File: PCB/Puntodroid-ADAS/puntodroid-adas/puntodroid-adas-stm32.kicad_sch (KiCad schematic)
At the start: 23 parts, among them J1 USB_B, J2 BOOTLOADER, J3 SWD PROGRAMMER, U1 STM32F446VETx, U2 CM1293A, Y1 16MHz

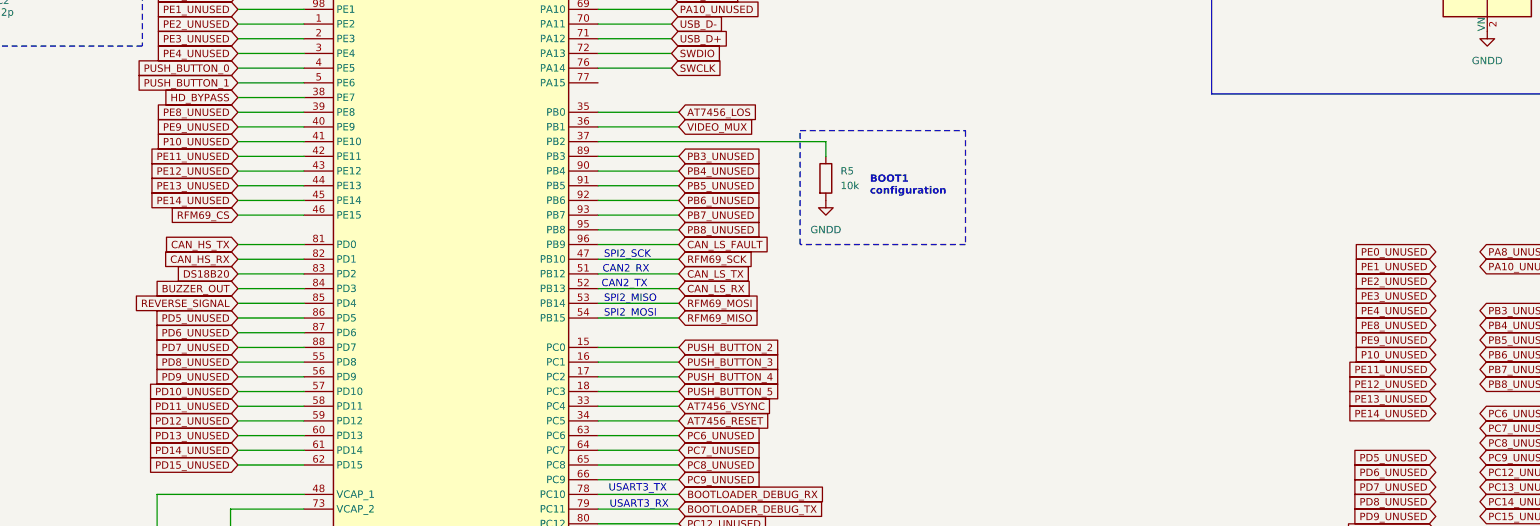
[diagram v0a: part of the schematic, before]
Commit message: update puntodroid schematic
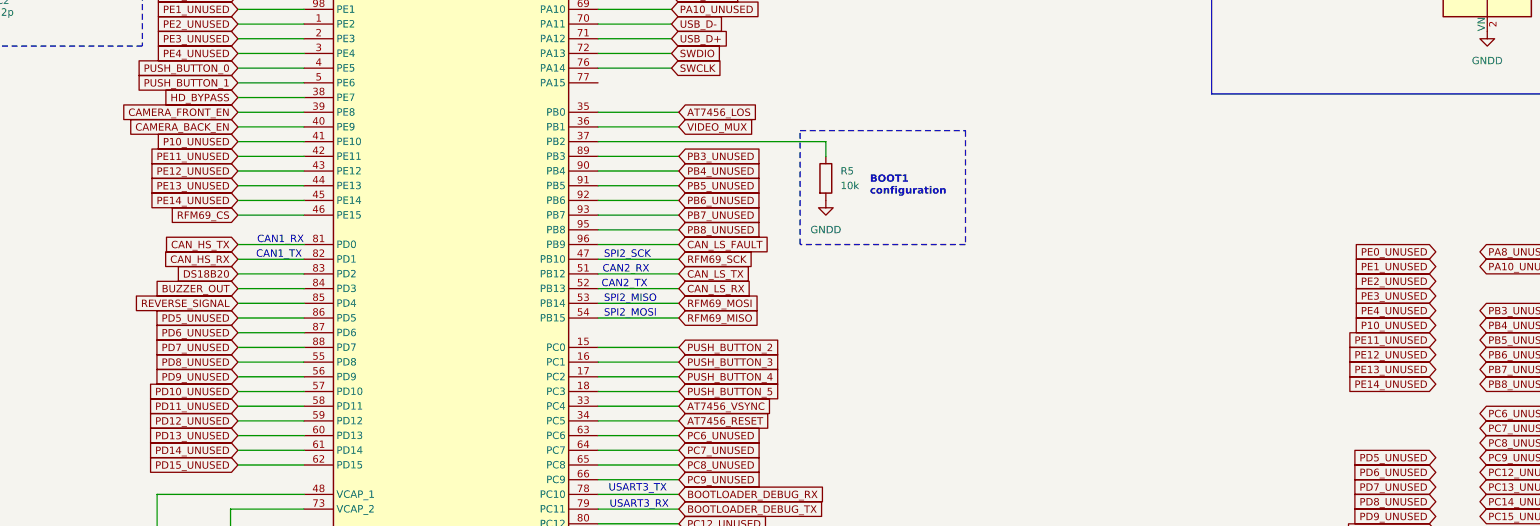
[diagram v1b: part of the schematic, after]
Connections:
- net PE8_UNUSED renamed CAMERA_FRONT_EN
- net PE9_UNUSED renamed CAMERA_BACK_EN
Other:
- note added: "CAN1_RX"
- note added: "CAN1_TX"
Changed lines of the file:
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@@
 		)
 	)
+	(text "CAN1_RX"
+		(exclude_from_sim no)
+		(at 157.226 128.778 0)
+		(effects
+			(font
+				(size 1.27 1.27)
+			)
+		)
+	)
+	(text "CAN1_TX"
+		(exclude_from_sim no)
+		(at 156.972 131.318 0)
+		(effects
+			(font
+				(size 1.27 1.27)
+			)
+		)
+	)
 	(text "USB SOCKET"
 		(exclude_from_sim no)
@@
 		)
 	)
-	(global_label "PE8_UNUSED"
+	(global_label "USB_D+"
 		(shape input)
-		(at 356.87 143.51 180)
+		(at 384.81 52.07 0)
 		(fields_autoplaced yes)
 		(effects
 			(font
 				(size 1.27 1.27)
-				(thickness 0.1588)
-				(color 255 0 255 1)
 			)
-			(justify right)
+			(justify left)
 		)
 		(property "Intersheetrefs" "${INTERSHEET_REFS}"
-			(at 341.1927 143.51 0)
+			(at 395.4152 52.07 0)
 			(effects
 				(font
 					(size 1.27 1.27)
 				)
-				(justify right)
+				(justify left)
 				(hide yes)
 			)
 		)
 	)
-	(global_label "USB_D+"
+	(global_label "CAMERA_FRONT_EN"
 		(shape input)
-		(at 384.81 52.07 0)
+		(at 149.86 106.68 180)
 		(fields_autoplaced yes)
 		(effects
@@
 				(size 1.27 1.27)
 			)
-			(justify left)
+			(justify right)
 		)
 		(property "Intersheetrefs" "${INTERSHEET_REFS}"
-			(at 395.4152 52.07 0)
+			(at 136.1705 106.68 0)
 			(effects
 				(font
 					(size 1.27 1.27)
 				)
-				(justify left)
+				(justify right)
 				(hide yes)
 			)
@@
 		)
 	)
-	(global_label "PE9_UNUSED"
-		(shape input)
-		(at 356.87 146.05 180)
-		(fields_autoplaced yes)
-		(effects
-			(font
-				(size 1.27 1.27)
-				(thickness 0.1588)
-				(color 255 0 255 1)
-			)
-			(justify right)
-		)
-		(property "Intersheetrefs" "${INTERSHEET_REFS}"
-			(at 341.1927 146.05 0)
-			(effects
-				(font
-					(size 1.27 1.27)
-				)
-				(justify right)
-				(hide yes)
-			)
-		)
-	)
 	(global_label "PD14_UNUSED"
 		(shape input)
@@
 		)
 	)
-	(global_label "PE8_UNUSED"
-		(shape input)
-		(at 149.86 106.68 180)
-		(fields_autoplaced yes)
-		(effects
-			(font
-				(size 1.27 1.27)
-				(thickness 0.1588)
-				(color 255 0 255 1)
-			)
-			(justify right)
-		)
-		(property "Intersheetrefs" "${INTERSHEET_REFS}"
-			(at 134.1827 106.68 0)
-			(effects
-				(font
-					(size 1.27 1.27)
-				)
-				(justify right)
-				(hide yes)
-			)
-		)
-	)
 	(global_label "PE1_UNUSED"
 		(shape input)
@@
 	(global_label "PE14_UNUSED"
 		(shape input)
-		(at 356.87 158.75 180)
+		(at 356.87 153.67 180)
 		(fields_autoplaced yes)
 		(effects
@@
 		)
 		(property "Intersheetrefs" "${INTERSHEET_REFS}"
-			(at 341.1927 158.75 0)
+			(at 341.1927 153.67 0)
 			(effects
 				(font
@@
 	(global_label "P10_UNUSED"
 		(shape input)
-		(at 356.87 148.59 180)
+		(at 356.87 143.51 180)
 		(fields_autoplaced yes)
 		(effects
@@
 		)
 		(property "Intersheetrefs" "${INTERSHEET_REFS}"
-			(at 341.1927 148.59 0)
+			(at 341.1927 143.51 0)
 			(effects
 				(font
@@
 		)
 	)
-	(global_label "PE9_UNUSED"
-		(shape input)
-		(at 149.86 109.22 180)
-		(fields_autoplaced yes)
-		(effects
-			(font
-				(size 1.27 1.27)
-				(thickness 0.1588)
-				(color 255 0 255 1)
-			)
-			(justify right)
-		)
-		(property "Intersheetrefs" "${INTERSHEET_REFS}"
-			(at 134.1827 109.22 0)
-			(effects
-				(font
-					(size 1.27 1.27)
-				)
-				(justify right)
-				(hide yes)
-			)
-		)
-	)
 	(global_label "PA8_UNUSED"
 		(shape input)
@@
 	(global_label "PE13_UNUSED"
 		(shape input)
-		(at 356.87 156.21 180)
+		(at 356.87 151.13 180)
 		(fields_autoplaced yes)
 		(effects
@@
 		)
 		(property "Intersheetrefs" "${INTERSHEET_REFS}"
-			(at 341.1927 156.21 0)
+			(at 341.1927 151.13 0)
 			(effects
 				(font
@@
 		)
 	)
+	(global_label "CAMERA_BACK_EN"
+		(shape input)
+		(at 149.86 109.22 180)
+		(fields_autoplaced yes)
+		(effects
+			(font
+				(size 1.27 1.27)
+			)
+			(justify right)
+		)
+		(property "Intersheetrefs" "${INTERSHEET_REFS}"
+			(at 130.2439 109.22 0)
+			(effects
+				(font
+					(size 1.27 1.27)
+				)
+				(justify right)
+				(hide yes)
+			)
+		)
+	)
 	(global_label "PC12_UNUSED"
 		(shape input)
@@
 	(global_label "PE12_UNUSED"
 		(shape input)
-		(at 356.87 153.67 180)
+		(at 356.87 148.59 180)
 		(fields_autoplaced yes)
 		(effects
@@
 		)
 		(property "Intersheetrefs" "${INTERSHEET_REFS}"
-			(at 341.1927 153.67 0)
+			(at 341.1927 148.59 0)
 			(effects
 				(font
@@
 	(global_label "PE11_UNUSED"
 		(shape input)
-		(at 356.87 151.13 180)
+		(at 356.87 146.05 180)
 		(fields_autoplaced yes)
 		(effects
@@
 		)
 		(property "Intersheetrefs" "${INTERSHEET_REFS}"
-			(at 341.1927 151.13 0)
+			(at 341.1927 146.05 0)
 			(effects
 				(font

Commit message: update puntodroid schematic stm32
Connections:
- net PA15_UNUSED: now reaches U1.77 (PA15)
- net PD5_UNUSED renamed ANDROID_EN
- net PE14_UNUSED renamed RFM69_RESET
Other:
- note added: "STM32F446 MICROCONTROLLER"
- moved on the sheet: C10, C12, C13, C5, C6, C7, C8, C9
